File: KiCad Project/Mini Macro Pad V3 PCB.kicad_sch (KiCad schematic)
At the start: 27 parts, among them J1 USB_C_Receptacle_USB2.0_14P, SW1 SW_Push bootsel, U1 RP2040, U2 NCP1117-3.3_SOT223, U3 W25Q128JVS

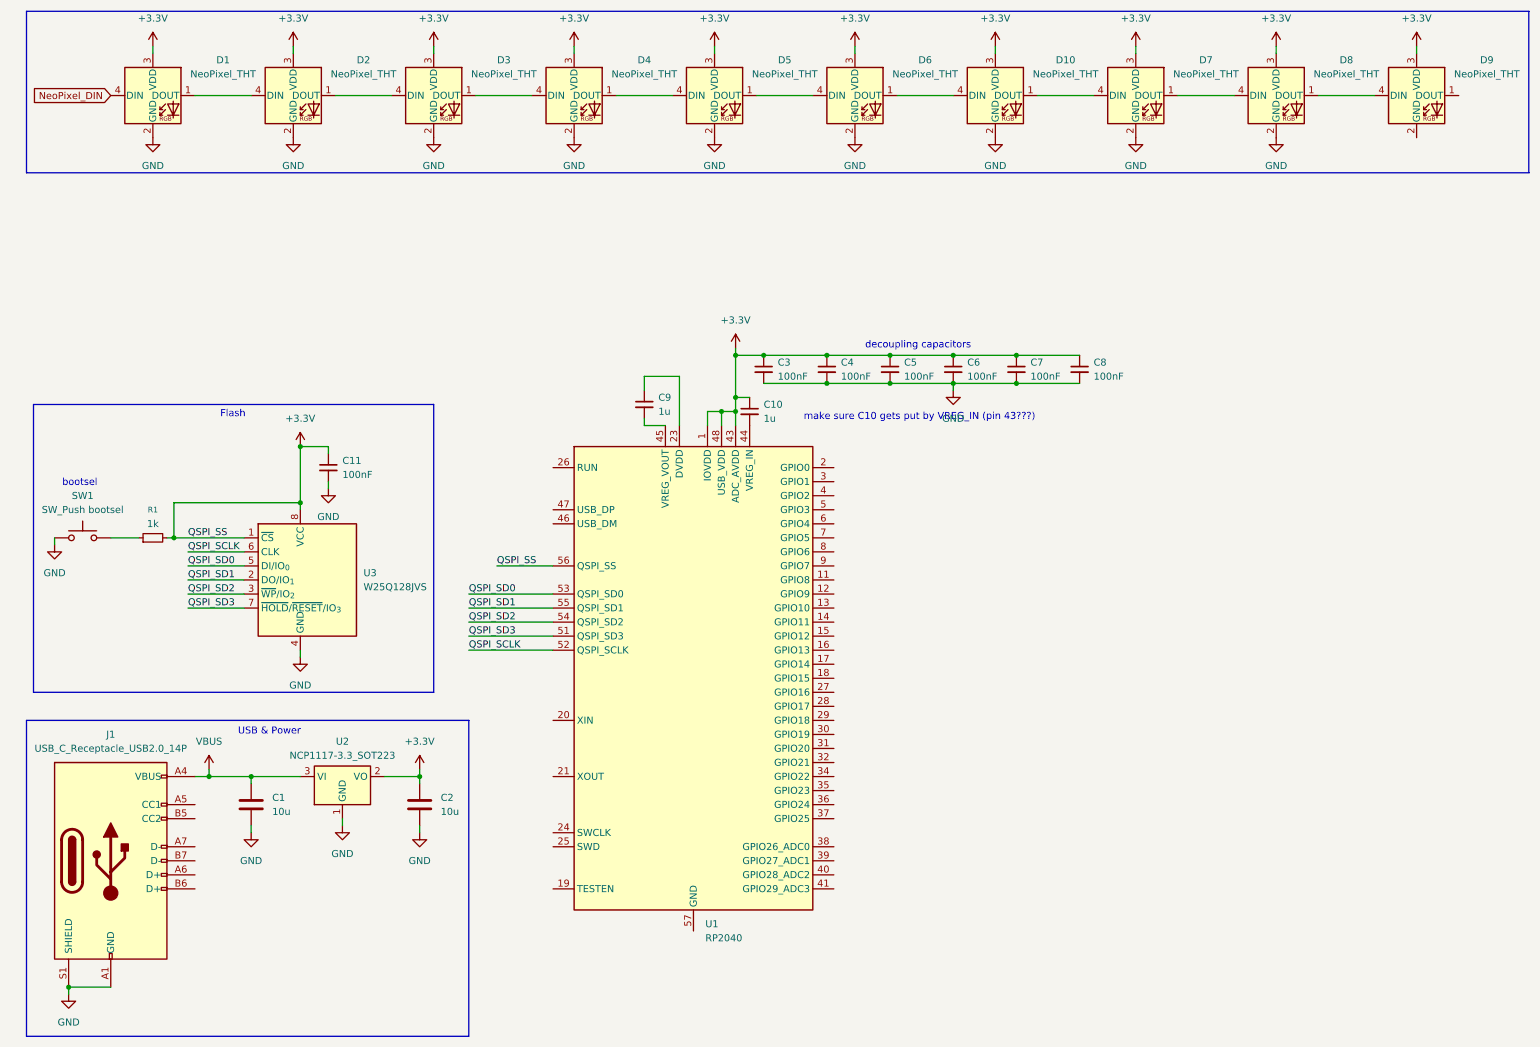
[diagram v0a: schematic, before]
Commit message: added crystal to schematic
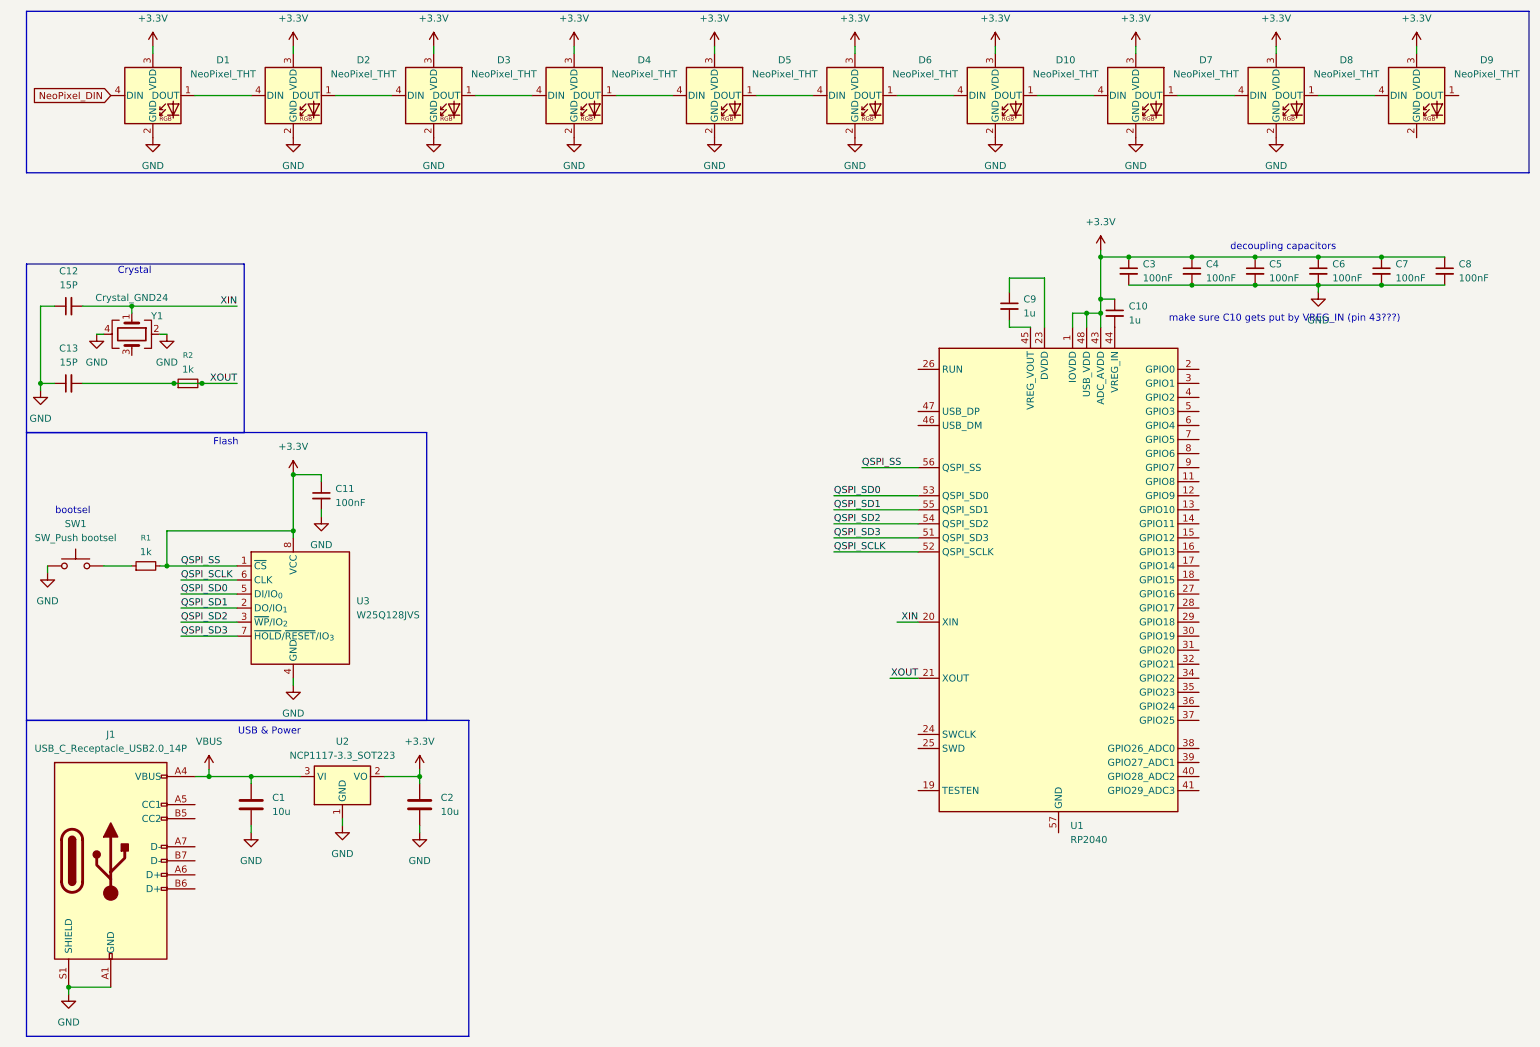
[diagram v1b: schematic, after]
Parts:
- added C12, C13: 15P, symbol Device:C_Small
- added R2: 1k, symbol Device:R_Small
- added Y1: Crystal_GND24, symbol Device:Crystal_GND24
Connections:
- net GND: now also C12.1, C13.1, Y1.2, Y1.4
- net XIN: now reaches U1.20 (XIN)
- net XIN: now also C12.2, Y1.1
- net XOUT: now reaches U1.21 (XOUT)
- net XOUT: now also C13.2, R2.1, R2.2
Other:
- note added: "Crystal"
- moved on the sheet: C10, C11, C3, C4, C5, C6, C7, C8, C9, R1, SW1, U1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
